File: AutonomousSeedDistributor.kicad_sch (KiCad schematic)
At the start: 0 parts

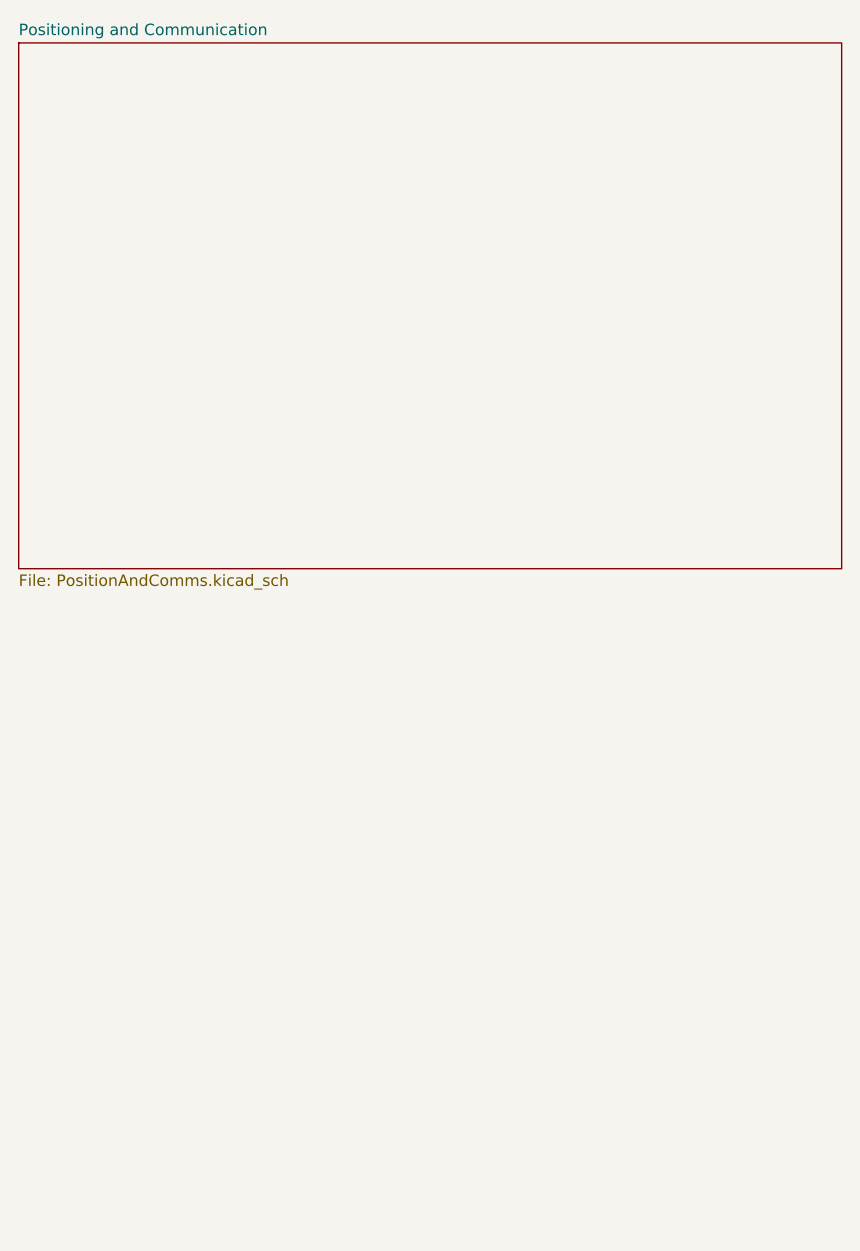
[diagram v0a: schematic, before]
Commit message: schematics for subsystem mostly done
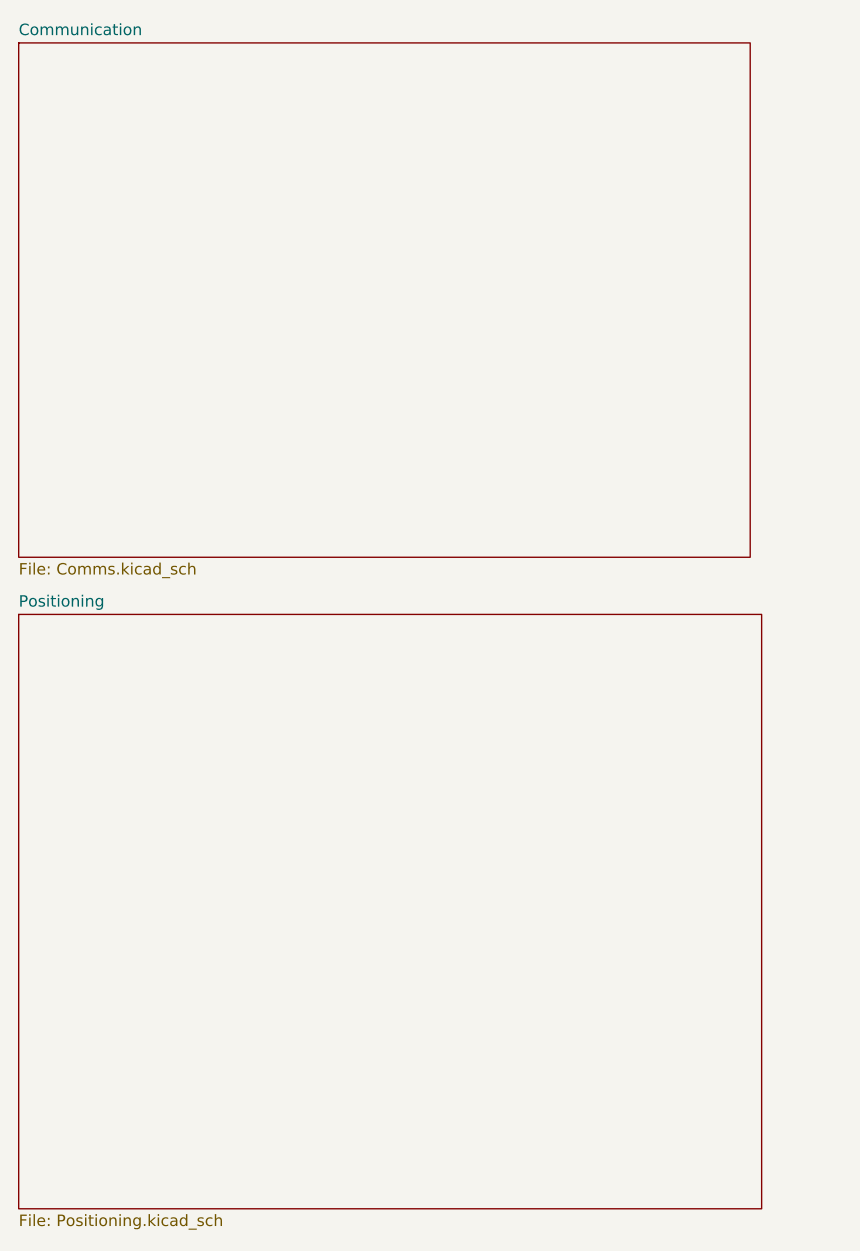
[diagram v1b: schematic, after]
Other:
- sheet Positioning and Communication renamed Communication
- added sheet Positioning (Positioning.kicad_sch)
- sheet Communication: file PositionAndComms.kicad_sch -> Comms.kicad_sch
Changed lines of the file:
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@@
 	(paper "A4")
 	(sheet
-		(at 20.32 24.13)
-		(size 91.44 58.42)
+		(at 20.32 87.63)
+		(size 82.55 66.04)
 		(fields_autoplaced yes)
 		(stroke
@@
 			(color 0 0 0 0.0000)
 		)
-		(property "Sheetname" "Positioning and Communication"
+		(property "Sheetname" "Positioning"
+			(at 20.32 86.9184 0)
+			(effects
+				(font
+					(size 1.27 1.27)
+				)
+				(justify left bottom)
+			)
+		)
+		(property "Sheetfile" "Positioning.kicad_sch"
+			(at 20.32 154.2546 0)
+			(effects
+				(font
+					(size 1.27 1.27)
+				)
+				(justify left top)
+			)
+		)
+		(instances
+			(project "AutonomousSeedDistributor"
+				(path "/2f4a034c-8d2d-4528-8fc9-76e665033073"
+					(page "3")
+				)
+			)
+		)
+	)
+	(sheet
+		(at 20.32 24.13)
+		(size 81.28 57.15)
+		(fields_autoplaced yes)
+		(stroke
+			(width 0.1524)
+			(type solid)
+		)
+		(fill
+			(color 0 0 0 0.0000)
+		)
+		(property "Sheetname" "Communication"
 			(at 20.32 23.4184 0)
 			(effects
@@
 			)
 		)
-		(property "Sheetfile" "PositionAndComms.kicad_sch"
-			(at 20.32 83.1346 0)
+		(property "Sheetfile" "Comms.kicad_sch"
+			(at 20.32 81.8646 0)
 			(effects
 				(font

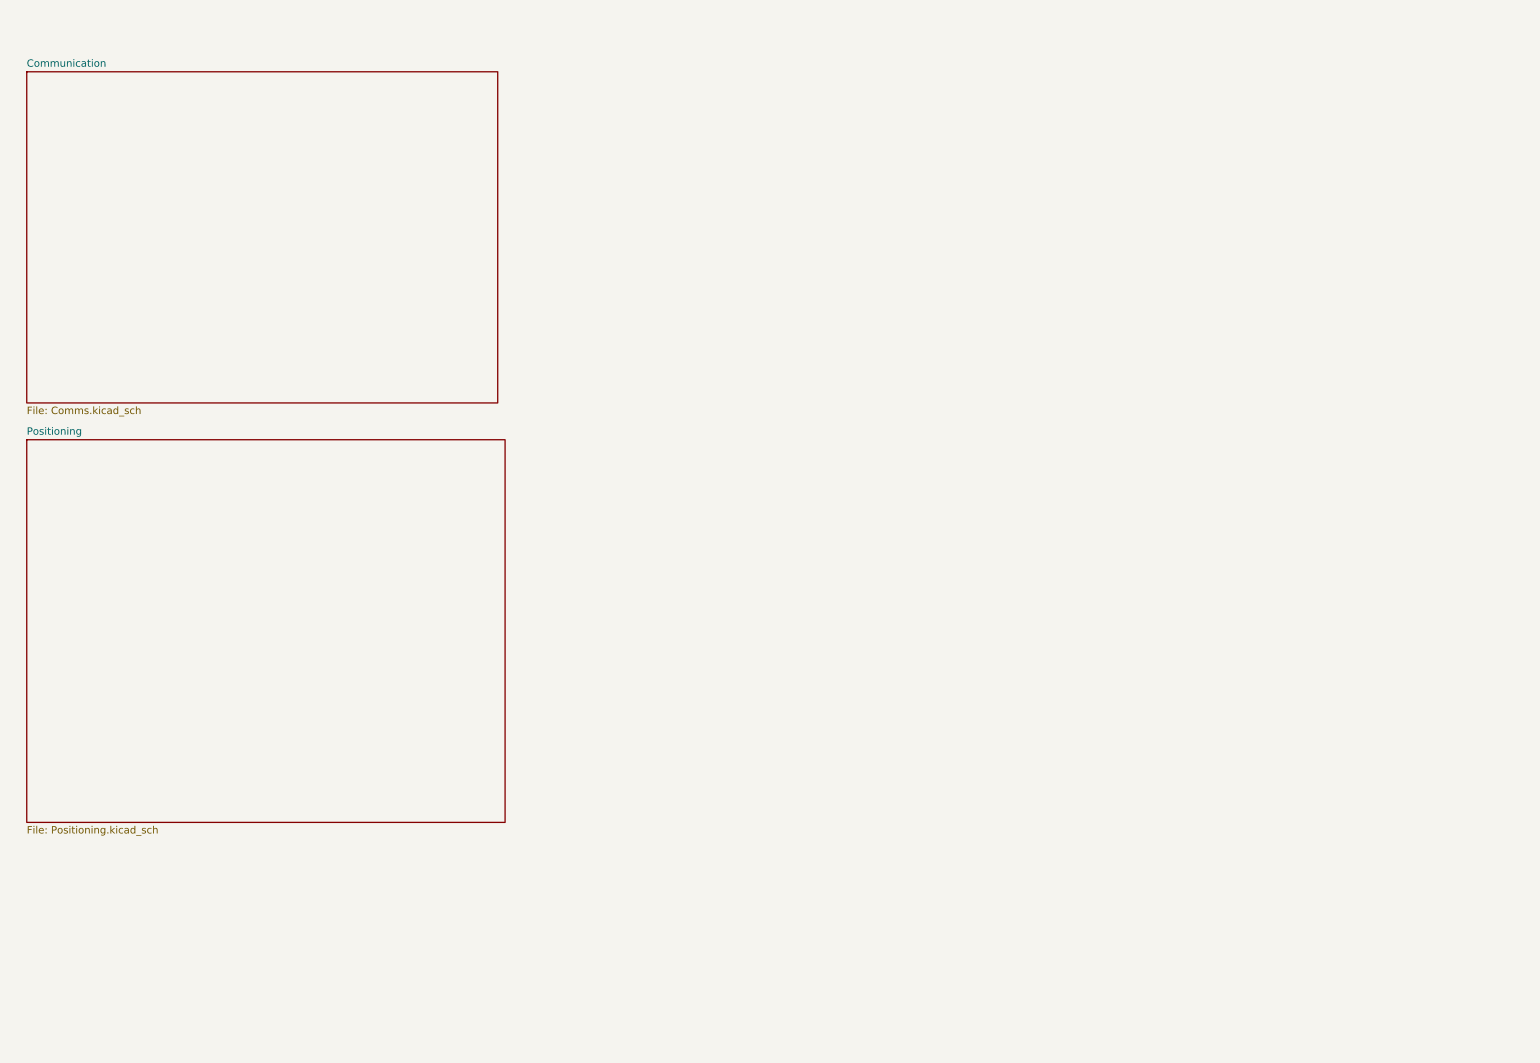
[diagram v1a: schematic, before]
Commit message: combined, submitted for Packaging Review
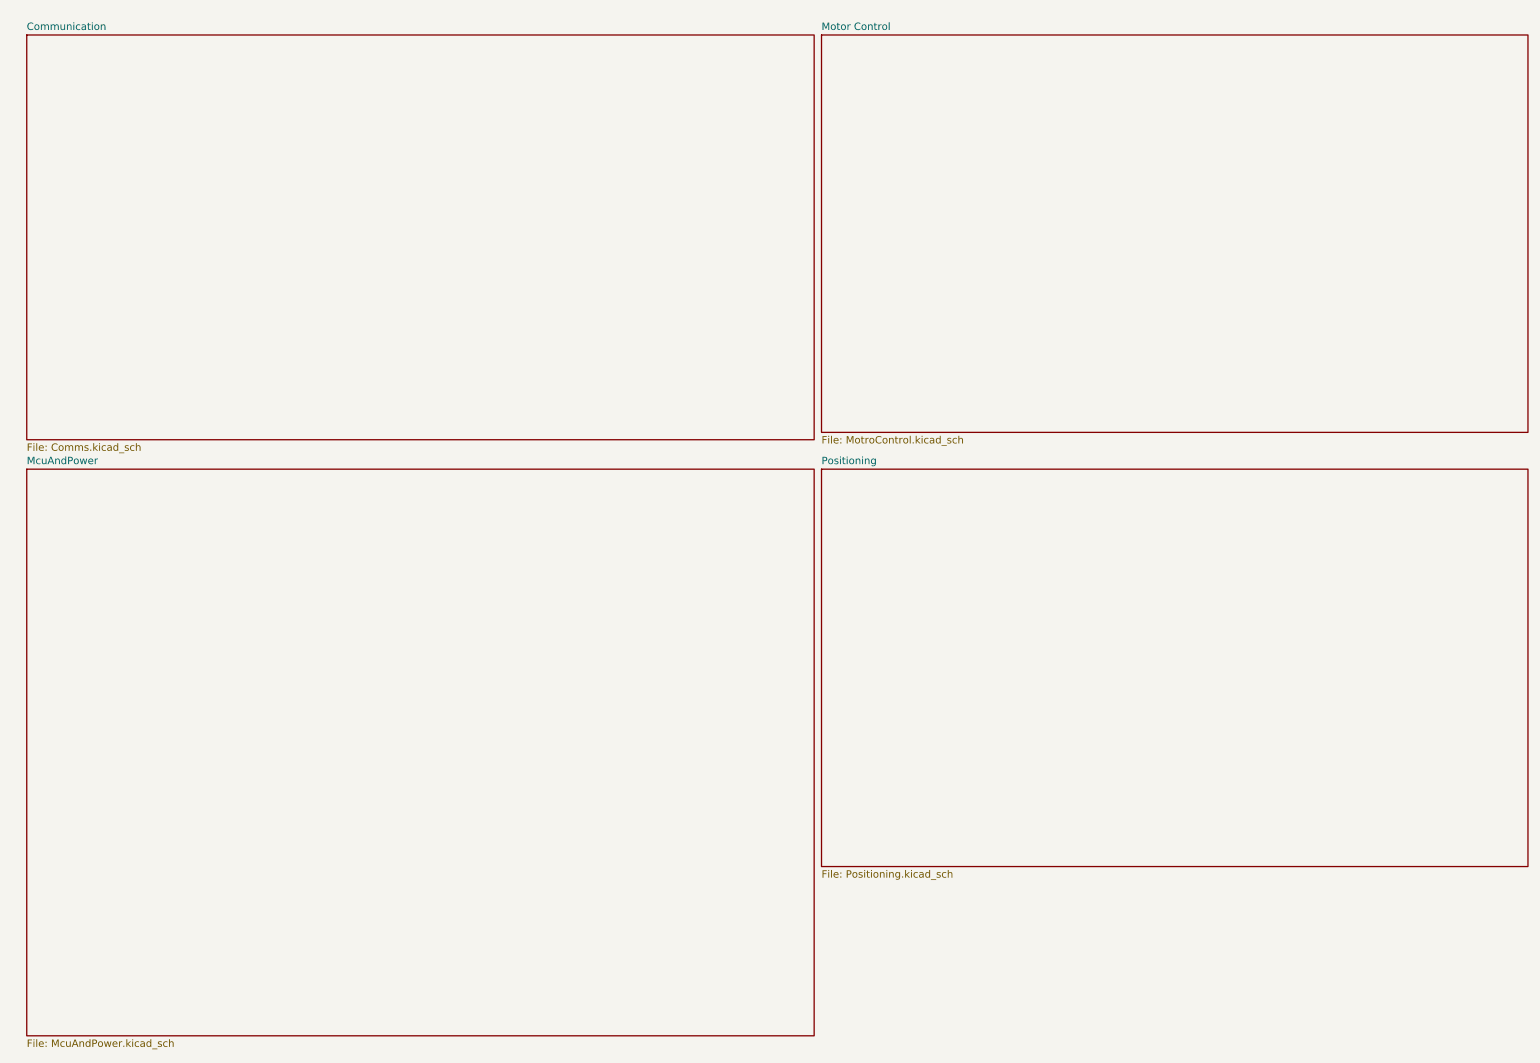
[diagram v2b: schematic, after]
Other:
- added sheet McuAndPower (McuAndPower.kicad_sch)
- added sheet Motor Control (MotroControl.kicad_sch)
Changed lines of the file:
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@@
 (kicad_sch
-	(version 20231120)
+	(version 20250114)
 	(generator "eeschema")
-	(generator_version "8.0")
+	(generator_version "9.0")
 	(paper "A4")
 	(sheet
-		(at 20.32 87.63)
-		(size 82.55 66.04)
+		(at 20.32 92.71)
+		(size 135.89 97.79)
+		(exclude_from_sim no)
+		(in_bom yes)
+		(on_board yes)
+		(dnp no)
+		(fields_autoplaced yes)
+		(stroke
+			(width 0.1524)
+			(type solid)
+		)
+		(fill
+			(color 0 0 0 0.0000)
+		)
+		(property "Sheetname" "McuAndPower"
+			(at 20.32 91.9984 0)
+			(effects
+				(font
+					(size 1.27 1.27)
+				)
+				(justify left bottom)
+			)
+		)
+		(property "Sheetfile" "McuAndPower.kicad_sch"
+			(at 20.32 191.0846 0)
+			(effects
+				(font
+					(size 1.27 1.27)
+				)
+				(justify left top)
+			)
+		)
+		(instances
+			(project "AutonomousSeedDistributor"
+				(path "/2f4a034c-8d2d-4528-8fc9-76e665033073"
+					(page "5")
+				)
+			)
+		)
+	)
+	(sheet
+		(at 157.48 92.71)
+		(size 121.92 68.58)
+		(exclude_from_sim no)
+		(in_bom yes)
+		(on_board yes)
+		(dnp no)
 		(fields_autoplaced yes)
 		(stroke
@@
 		)
 		(property "Sheetname" "Positioning"
-			(at 20.32 86.9184 0)
+			(at 157.48 91.9984 0)
 			(effects
 				(font
@@
 		)
 		(property "Sheetfile" "Positioning.kicad_sch"
-			(at 20.32 154.2546 0)
+			(at 157.48 161.8746 0)
 			(effects
 				(font
@@
 	)
 	(sheet
-		(at 20.32 24.13)
-		(size 81.28 57.15)
+		(at 20.32 17.78)
+		(size 135.89 69.85)
+		(exclude_from_sim no)
+		(in_bom yes)
+		(on_board yes)
+		(dnp no)
 		(fields_autoplaced yes)
 		(stroke
@@
 		)
 		(property "Sheetname" "Communication"
-			(at 20.32 23.4184 0)
+			(at 20.32 17.0684 0)
 			(effects
 				(font
@@
 		)
 		(property "Sheetfile" "Comms.kicad_sch"
-			(at 20.32 81.8646 0)
+			(at 20.32 88.2146 0)
 			(effects
 				(font
@@
 		)
 	)
+	(sheet
+		(at 157.48 17.78)
+		(size 121.92 68.58)
+		(exclude_from_sim no)
+		(in_bom yes)
+		(on_board yes)
+		(dnp no)
+		(fields_autoplaced yes)
+		(stroke
+			(width 0.1524)
+			(type solid)
+		)
+		(fill
+			(color 0 0 0 0.0000)
+		)
+		(property "Sheetname" "Motor Control"
+			(at 157.48 17.0684 0)
+			(effects
+				(font
+					(size 1.27 1.27)
+				)
+				(justify left bottom)
+			)
+		)
+		(property "Sheetfile" "MotroControl.kicad_sch"
+			(at 157.48 86.9446 0)
+			(effects
+				(font
+					(size 1.27 1.27)
+				)
+				(justify left top)
+			)
+		)
+		(instances
+			(project "AutonomousSeedDistributor"
+				(path "/2f4a034c-8d2d-4528-8fc9-76e665033073"
+					(page "4")
+				)
+			)
+		)
+	)
 	(sheet_instances
 		(path "/"
@@
 		)
 	)
+	(embedded_fonts no)
 )

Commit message: rev 1
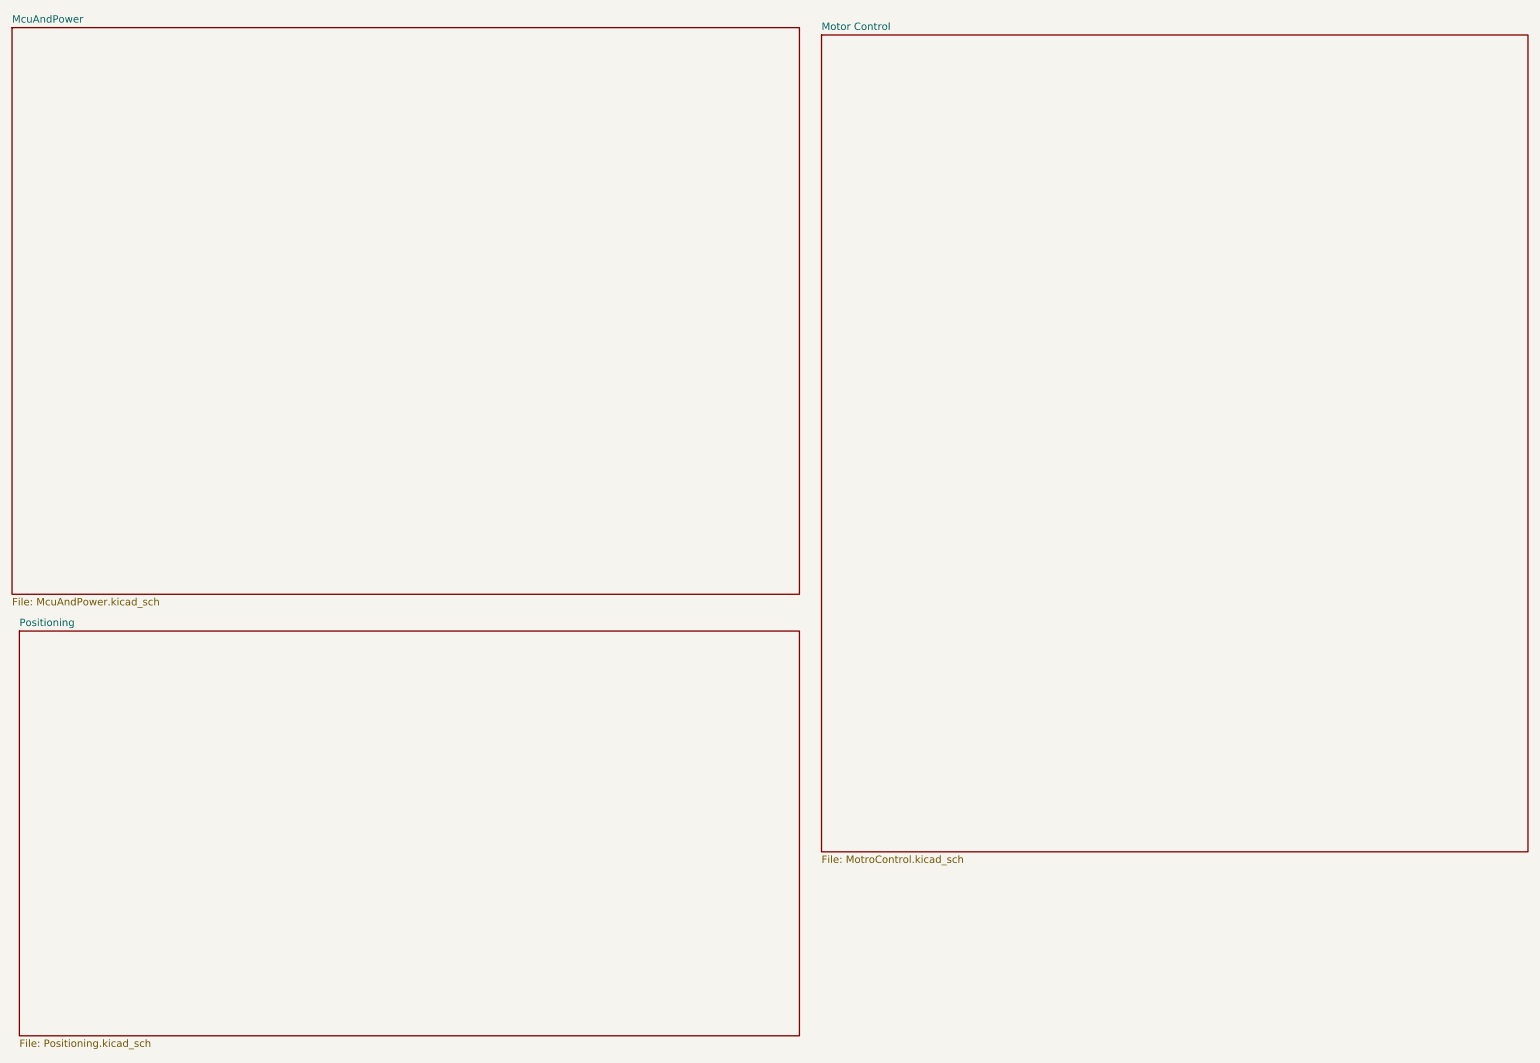
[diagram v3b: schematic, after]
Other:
- removed sheet Communication
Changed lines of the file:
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@@
 	(paper "A4")
 	(sheet
-		(at 20.32 92.71)
+		(at 17.78 16.51)
 		(size 135.89 97.79)
 		(exclude_from_sim no)
@@
 		)
 		(property "Sheetname" "McuAndPower"
-			(at 20.32 91.9984 0)
+			(at 17.78 15.7984 0)
 			(effects
 				(font
@@
 		)
 		(property "Sheetfile" "McuAndPower.kicad_sch"
-			(at 20.32 191.0846 0)
+			(at 17.78 114.8846 0)
 			(effects
 				(font
@@
 	)
 	(sheet
-		(at 157.48 92.71)
-		(size 121.92 68.58)
+		(at 19.05 120.65)
+		(size 134.62 69.85)
 		(exclude_from_sim no)
 		(in_bom yes)
@@
 		)
 		(property "Sheetname" "Positioning"
-			(at 157.48 91.9984 0)
+			(at 19.05 119.9384 0)
 			(effects
 				(font
@@
 		)
 		(property "Sheetfile" "Positioning.kicad_sch"
-			(at 157.48 161.8746 0)
+			(at 19.05 191.0846 0)
 			(effects
 				(font
@@
 	)
 	(sheet
-		(at 20.32 17.78)
-		(size 135.89 69.85)
-		(exclude_from_sim no)
-		(in_bom yes)
-		(on_board yes)
-		(dnp no)
-		(fields_autoplaced yes)
-		(stroke
-			(width 0.1524)
-			(type solid)
-		)
-		(fill
-			(color 0 0 0 0.0000)
-		)
-		(property "Sheetname" "Communication"
-			(at 20.32 17.0684 0)
-			(effects
-				(font
-					(size 1.27 1.27)
-				)
-				(justify left bottom)
-			)
-		)
-		(property "Sheetfile" "Comms.kicad_sch"
-			(at 20.32 88.2146 0)
-			(effects
-				(font
-					(size 1.27 1.27)
-				)
-				(justify left top)
-			)
-		)
-		(instances
-			(project "AutonomousSeedDistributor"
-				(path "/2f4a034c-8d2d-4528-8fc9-76e665033073"
-					(page "2")
-				)
-			)
-		)
-	)
-	(sheet
 		(at 157.48 17.78)
-		(size 121.92 68.58)
+		(size 121.92 140.97)
 		(exclude_from_sim no)
 		(in_bom yes)
@@
 		)
 		(property "Sheetfile" "MotroControl.kicad_sch"
-			(at 157.48 86.9446 0)
+			(at 157.48 159.3346 0)
 			(effects
 				(font
